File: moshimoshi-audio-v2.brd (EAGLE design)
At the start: 42.4 x 26.9 mm, 28 parts, among them IC1 LM386M-1, IC2 TL071D, IC3 INA134U

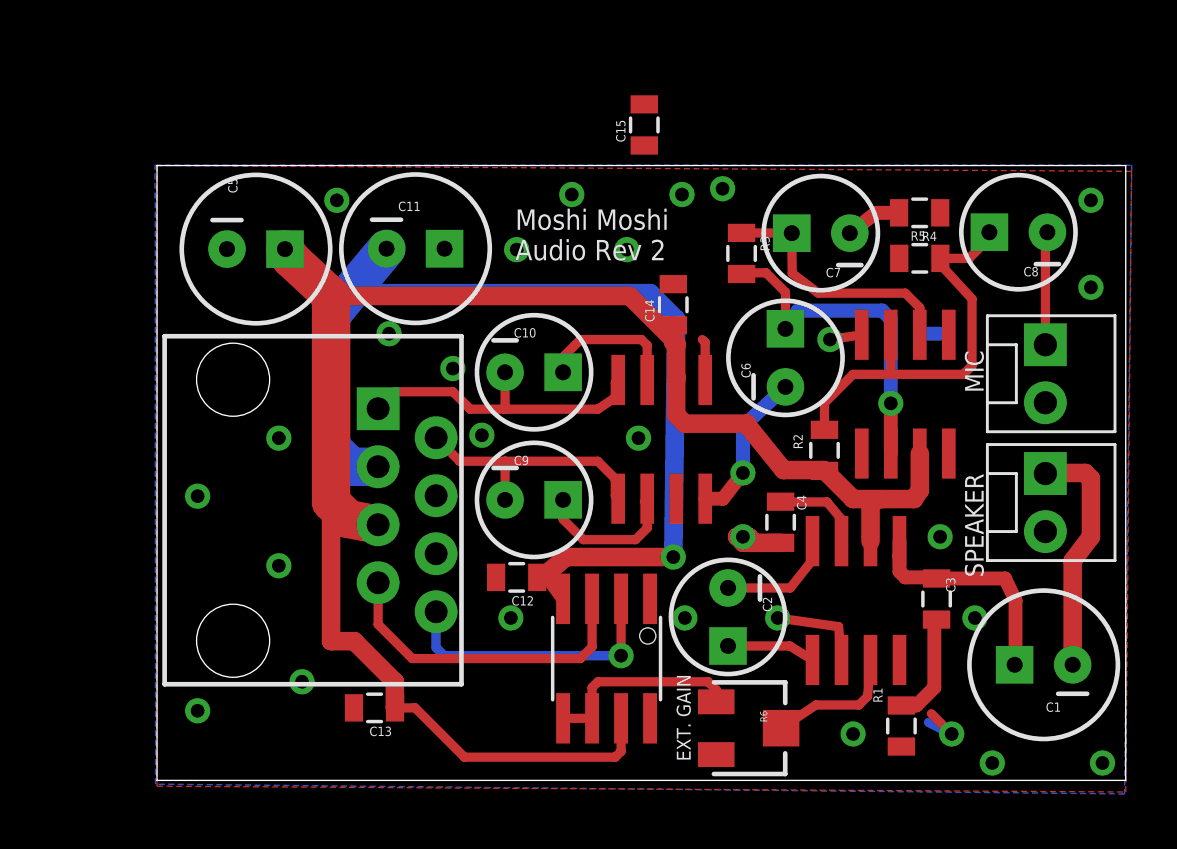
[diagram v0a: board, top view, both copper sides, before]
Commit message: Updated version with OW changes
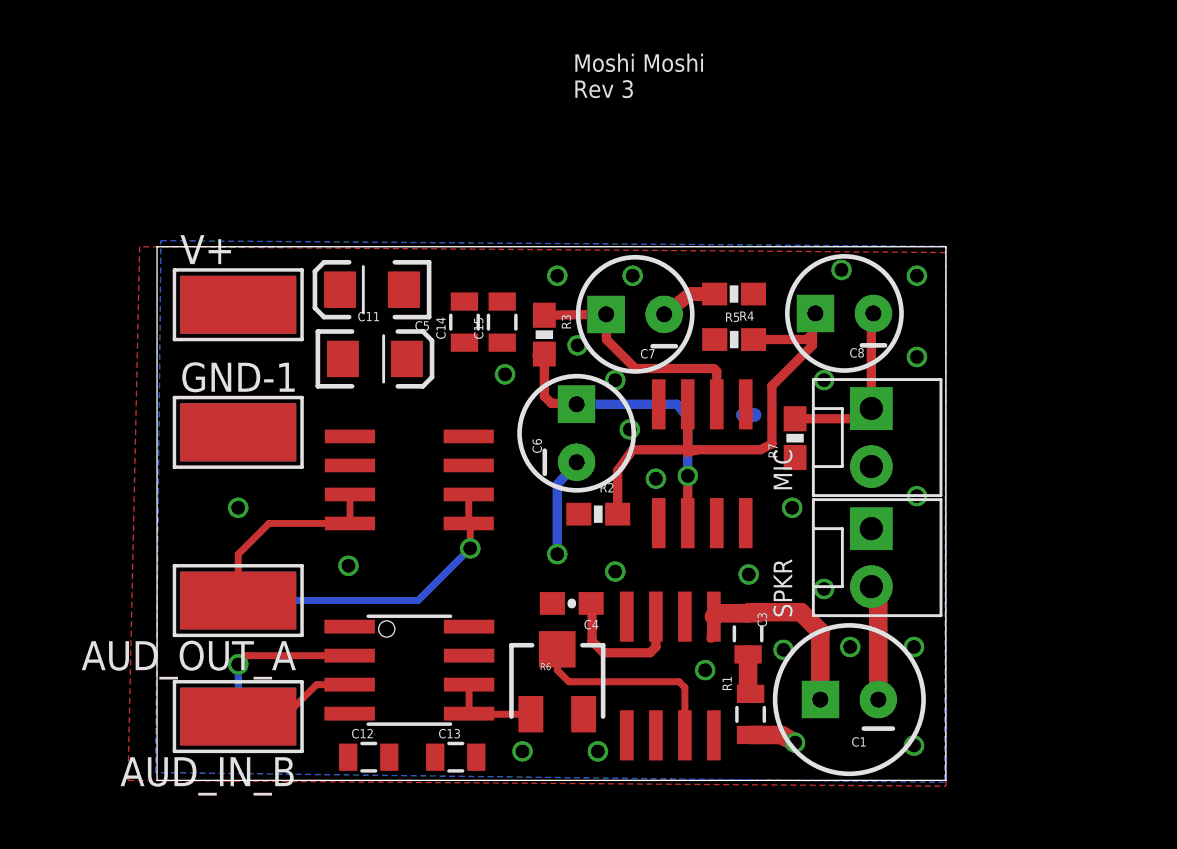
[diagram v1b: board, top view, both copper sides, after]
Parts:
- removed C10, C2, C9: 10uf, SparkFun-Capacitors:CPOL-RADIAL-10UF-25V
- removed JP1: RJ45, SparkFun-Connectors:RJ45-8
- removed U$1: DRV135UA, BurrBrownAudioParts:SO08
- added AUD_IN_A, AUD_IN_B, AUD_OUT_A, AUD_OUT_B, GND-1, GND-2, V+, V-: WIREPADSMD5-2,5, wirepad:5-2,5
- added IC4: DRV135UA, BurrBrownAudioParts:SO08
- added R7: 2K2, SparkFun-Resistors:0603-RES
- C11, C5: value 100uf -> 10uF; device SparkFun-Capacitors:CPOL-RADIAL-100UF-25V -> SparkFun-Capacitors:EIA3216
- C3: value 0.05uf -> 0.05uF
- C4: value 0.1uf -> 0.1uF; device SparkFun-Capacitors:0805 -> SparkFun-Capacitors:0603-CAP
- R1: value 10 -> 10R
- R2, R3, R4, R5: device SparkFun-Resistors:0805 -> SparkFun-Resistors:0603-RES
- moved C15 10.6 mm to (15.1, 20.1)
- moved R2 10.3 mm to (19.3, 11.7), turned to 180 degrees
- moved C12 10.2 mm to (9.27, 1.02), turned to 0 degrees
- moved C4 9.81 mm to (18.2, 7.75), turned to 180 degrees
- moved C6 9.72 mm to (18.4, 15.2)
- moved IC2 9.40 mm to (23.9, 13.9)
- moved R3 9.34 mm to (17.0, 19.5)
- moved C14 9.18 mm to (13.5, 20.1)
- moved R5 8.87 mm to (25.3, 19.3)
- moved C7 8.87 mm to (20.9, 20.4)
- moved R4 8.87 mm to (25.3, 21.3)
- moved IC1 8.77 mm to (22.5, 4.57)
- moved IC3 8.65 mm to (11.0, 4.83), turned to 270 degrees
- moved C1 8.64 mm to (30.3, 3.54)
- moved R6 8.62 mm to (17.5, 4.32), turned to 0 degrees
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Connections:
- removed net 15V-: C11.2, C12.1, C15.1, IC3.4, JP1.3, U$1.5
- removed net N$16: C9.1, U$1.2
- removed net N$17: C10.1, U$1.7
- removed net N$2: C2.2, IC1.8
- removed net N$7: C1.2, SPKR.1
- removed net VCC: C13.1, C14.1, C5.1, IC1.6, IC2.7, IC3.7, JP1.5, R2.2, U$1.6
- new net V+: C13.1, C14.1, C5.A, IC1.6, IC2.7, IC3.7, IC4.6, R2.2, R7.1, V+.1
- new net V-: C11.C, C12.1, C15.1, IC3.4, IC4.5, V-.1
- net A_OUT+: now also IC4.4; no longer U$1.4
- net GND: now also C11.A, C5.C, GND-1.1, GND-2.1, IC4.3, SPKR.1; no longer C11.1, C5.2, JP1.4, JP1.6, SPKR.2, U$1.3
- net IN+: now also AUD_IN_B.1; no longer JP1.7
- net IN-: now also AUD_IN_A.1; no longer JP1.8
- net MIC+: now also R7.2
- net N$1: now also C1.2, SPKR.2; no longer C2.1, IC1.1
- net OUT+: now also AUD_OUT_A.1, IC4.7, IC4.8; no longer C10.2, JP1.1, U$1.8
- net OUT-: now also AUD_OUT_B.1, IC4.1, IC4.2; no longer C9.2, JP1.2, U$1.1
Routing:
- net VCC: track 83.5 -> 0.00 mm
- net 15V-: track 46.4 -> 0.00 mm, vias 1 -> 0
- net N$7: track 10.5 -> 0.00 mm
- net GND: track 11.4 -> 2.55 mm, vias 28 -> 26
- net IN+: track 14.1 -> 6.16 mm
- net N$16: track 6.58 -> 0.00 mm
- net N$17: track 6.29 -> 0.00 mm
- net A_IN+: track 9.41 -> 3.99 mm
- net N$2: track 5.11 -> 0.00 mm
- net IN-: track 12.3 -> 7.32 mm
- net OUT+: track 13.6 -> 8.75 mm
- net N$3: track 5.85 -> 9.10 mm
- net N$6: track 4.78 -> 1.77 mm
- net N$11: track 18.1 -> 20.9 mm
- net MIC+: track 4.99 -> 7.70 mm
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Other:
- board size 42.4 x 26.9 mm -> 34.5 x 23.4 mm
- board text added: "Moshi Moshi Rev 3"
- board text added: "SPKR"
- board text removed: "EXT. GAIN"
- board text removed: "Moshi Moshi Audio Rev 2"
- board text removed: "SPEAKER"
